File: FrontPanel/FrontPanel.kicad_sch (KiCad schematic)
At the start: 66 parts, among them SW1 Channel 1, SW10 5, SW11 2, SW12 0, SW13 9, SW14 6, SW15 3, SW16 Backspace, SW17 Voltage 1, SW18 Current 1, SW19 Voltage 2, SW2 Confirm, SW20 Current 2, SW3 Cancel, SW4 Channel 2, SW5 7, SW6 4, SW7 1, SW8 Decimal, SW9 8

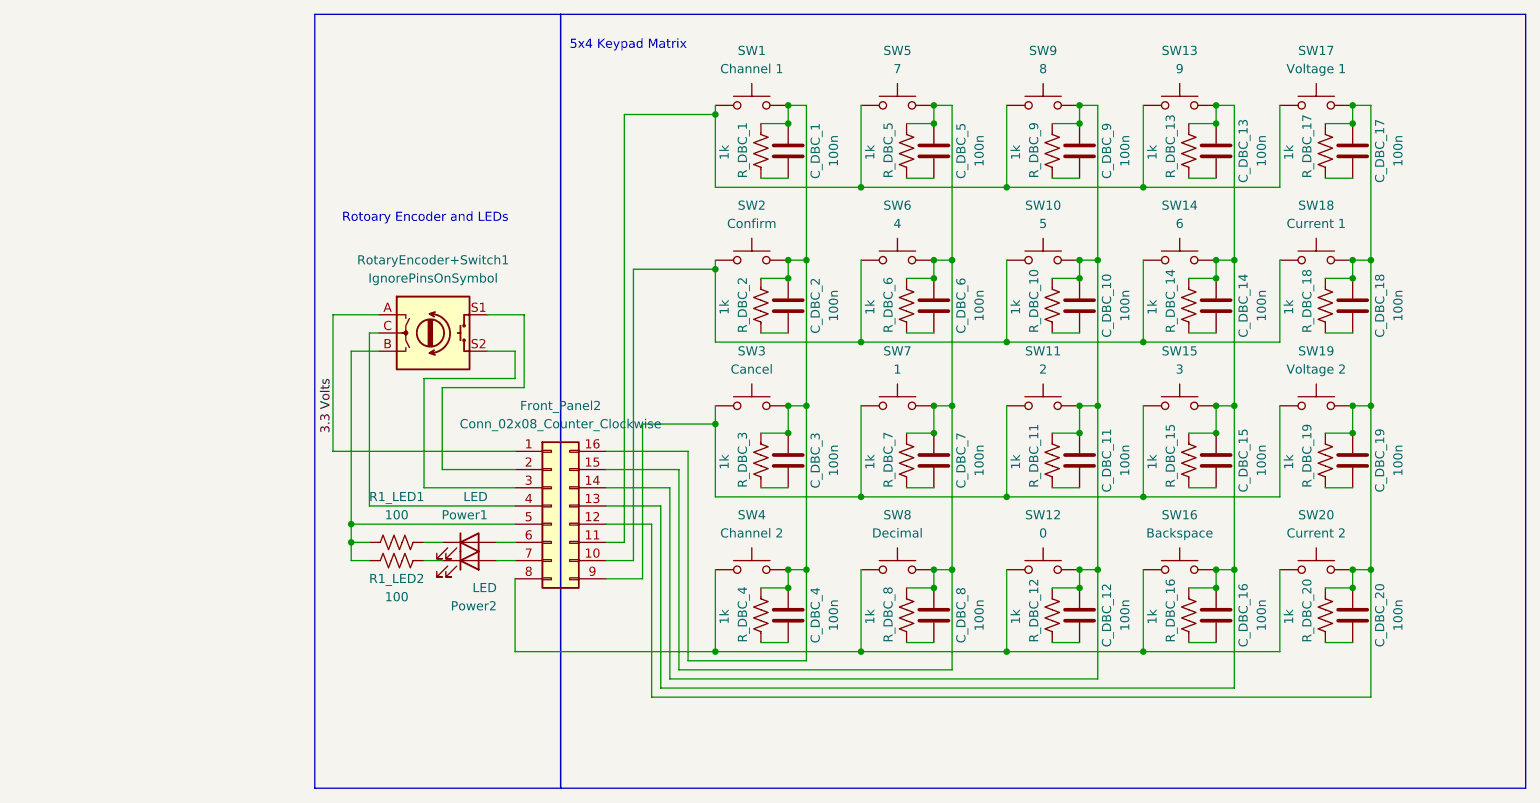
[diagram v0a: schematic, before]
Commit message: Front Panel
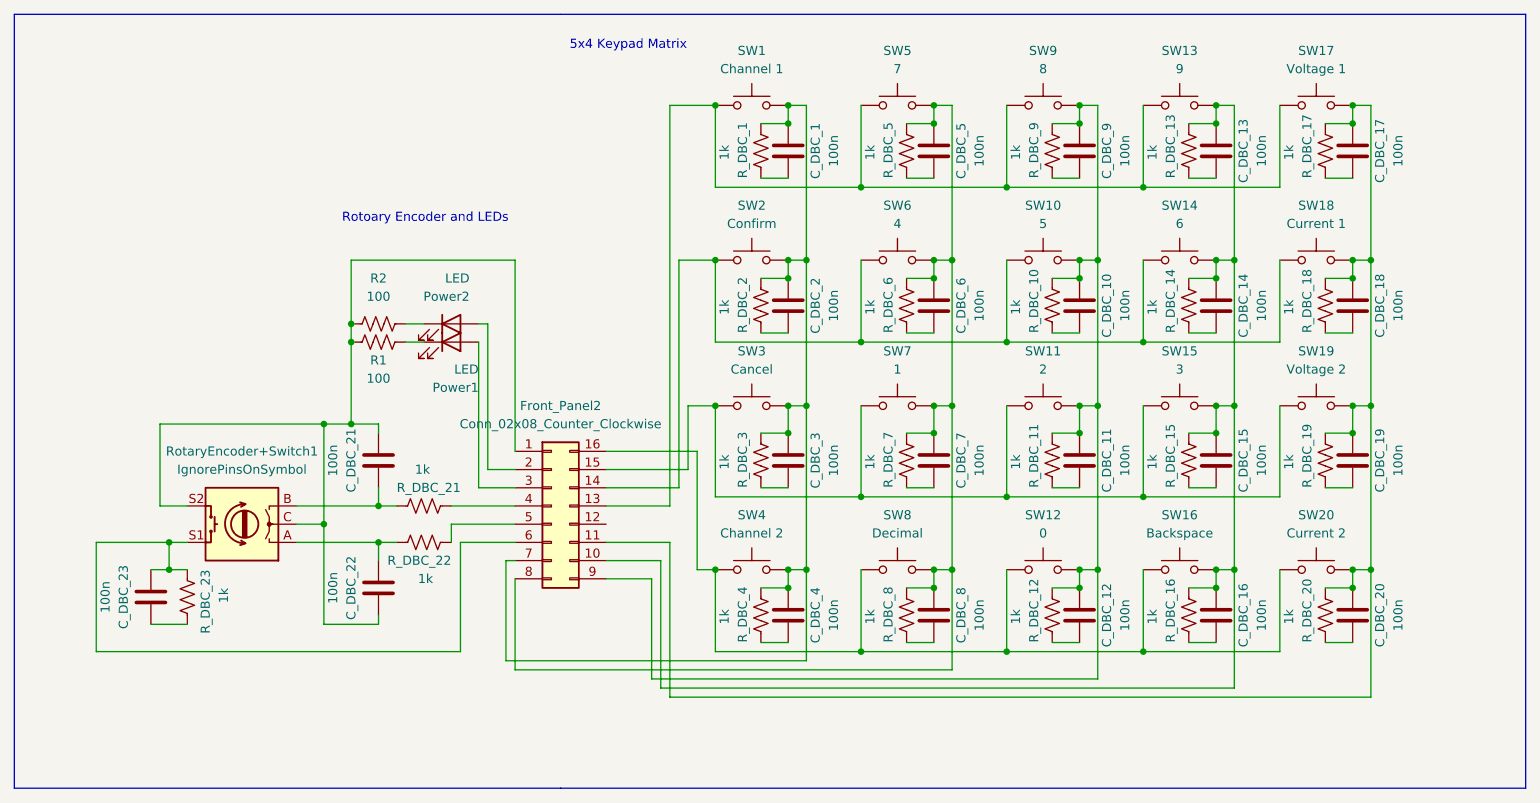
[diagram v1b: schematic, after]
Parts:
- added C_DBC_21, C_DBC_22, C_DBC_23: 100n, Capacitor_SMD:C_0603_1608Metric, symbol Device:C
- added R_DBC_21, R_DBC_22, R_DBC_23: 1k, Resistor_SMD:R_0603_1608Metric, symbol Device:R_US
- Power1: renamed from Power2; footprint LED_THT:LED_D3.0mm -> LED_SMD:LED_0603_1608Metric
- Power2: renamed from Power1; footprint LED_THT:LED_D3.0mm -> LED_SMD:LED_0603_1608Metric
- renumbered R1_LED2 to R1, R1_LED1 to R2
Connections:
- net at C_DBC_17.2, C_DBC_18.2, C_DBC_19.2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: now also Front_Panel2.11 (Pin_11); no longer Front_Panel2.12 (Pin_12)
- net at SW10.1, SW14.1, SW18.1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: now also Front_Panel2.14 (Pin_14); no longer Front_Panel2.10 (Pin_10)
- net at C_DBC_13.2, C_DBC_14.2, C_DBC_15.2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: now also Front_Panel2.10 (Pin_10); no longer Front_Panel2.13 (Pin_13)
- net at SW12.1, SW16.1, SW20.1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: now also Front_Panel2.16 (Pin_16); no longer Front_Panel2.8 (Pin_8)
- net at C_DBC_10.2, C_DBC_11.2, C_DBC_12.2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: now also Front_Panel2.9 (Pin_9); no longer Front_Panel2.14 (Pin_14)
- net at SW11.1, SW15.1, SW19.1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: now also Front_Panel2.15 (Pin_15); no longer Front_Panel2.9 (Pin_9)
- net at C_DBC_5.2, C_DBC_6.2, C_DBC_7.2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: now also Front_Panel2.8 (Pin_8); no longer Front_Panel2.15 (Pin_15)
- net at C_DBC_1.2, C_DBC_2.2, C_DBC_3.2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: now also Front_Panel2.7 (Pin_7); no longer Front_Panel2.16 (Pin_16)
- net at Power1.2 (A): now also Front_Panel2.3 (Pin_3); no longer Front_Panel2.7 (Pin_7)
- net at R1.2, R2.2: now also Front_Panel2.1 (Pin_1), RotaryEncoder+Switch1.C, RotaryEncoder+Switch1.S2, C_DBC_21.1, C_DBC_22.2; no longer Front_Panel2.5 (Pin_5), RotaryEncoder+Switch1.B
- net at SW1.1, SW13.1, SW17.1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: now also Front_Panel2.13 (Pin_13); no longer Front_Panel2.11 (Pin_11)
- net at RotaryEncoder+Switch1.S1: now also Front_Panel2.6 (Pin_6), C_DBC_23.1, R_DBC_23.2; no longer Front_Panel2.2 (Pin_2)
- net at Front_Panel2.4 (Pin_4): now also R_DBC_21.1; no longer RotaryEncoder+Switch1.C
- net at Power2.2 (A): now also Front_Panel2.2 (Pin_2); no longer Front_Panel2.6 (Pin_6)
- net 3.3 Volts: no longer names the net of RotaryEncoder+Switch1.A
- net 3.3 Volts: now also C_DBC_22.1, R_DBC_22.1; no longer Front_Panel2.1 (Pin_1)
- new net: C_DBC_23.2, R_DBC_23.1
- new net: C_DBC_21.2, R_DBC_21.2, RotaryEncoder+Switch1.B
- new net: Front_Panel2.5 (Pin_5), R_DBC_22.2
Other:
- moved on the sheet: Power1, Power2, R1, R2, RotaryEncoder+Switch1
